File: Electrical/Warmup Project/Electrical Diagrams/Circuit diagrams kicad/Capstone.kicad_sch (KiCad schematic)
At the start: 15 parts, among them M2 Motor_DC, U2 MCP2561-E-MF, U3 OP AMP, U4 INA125P

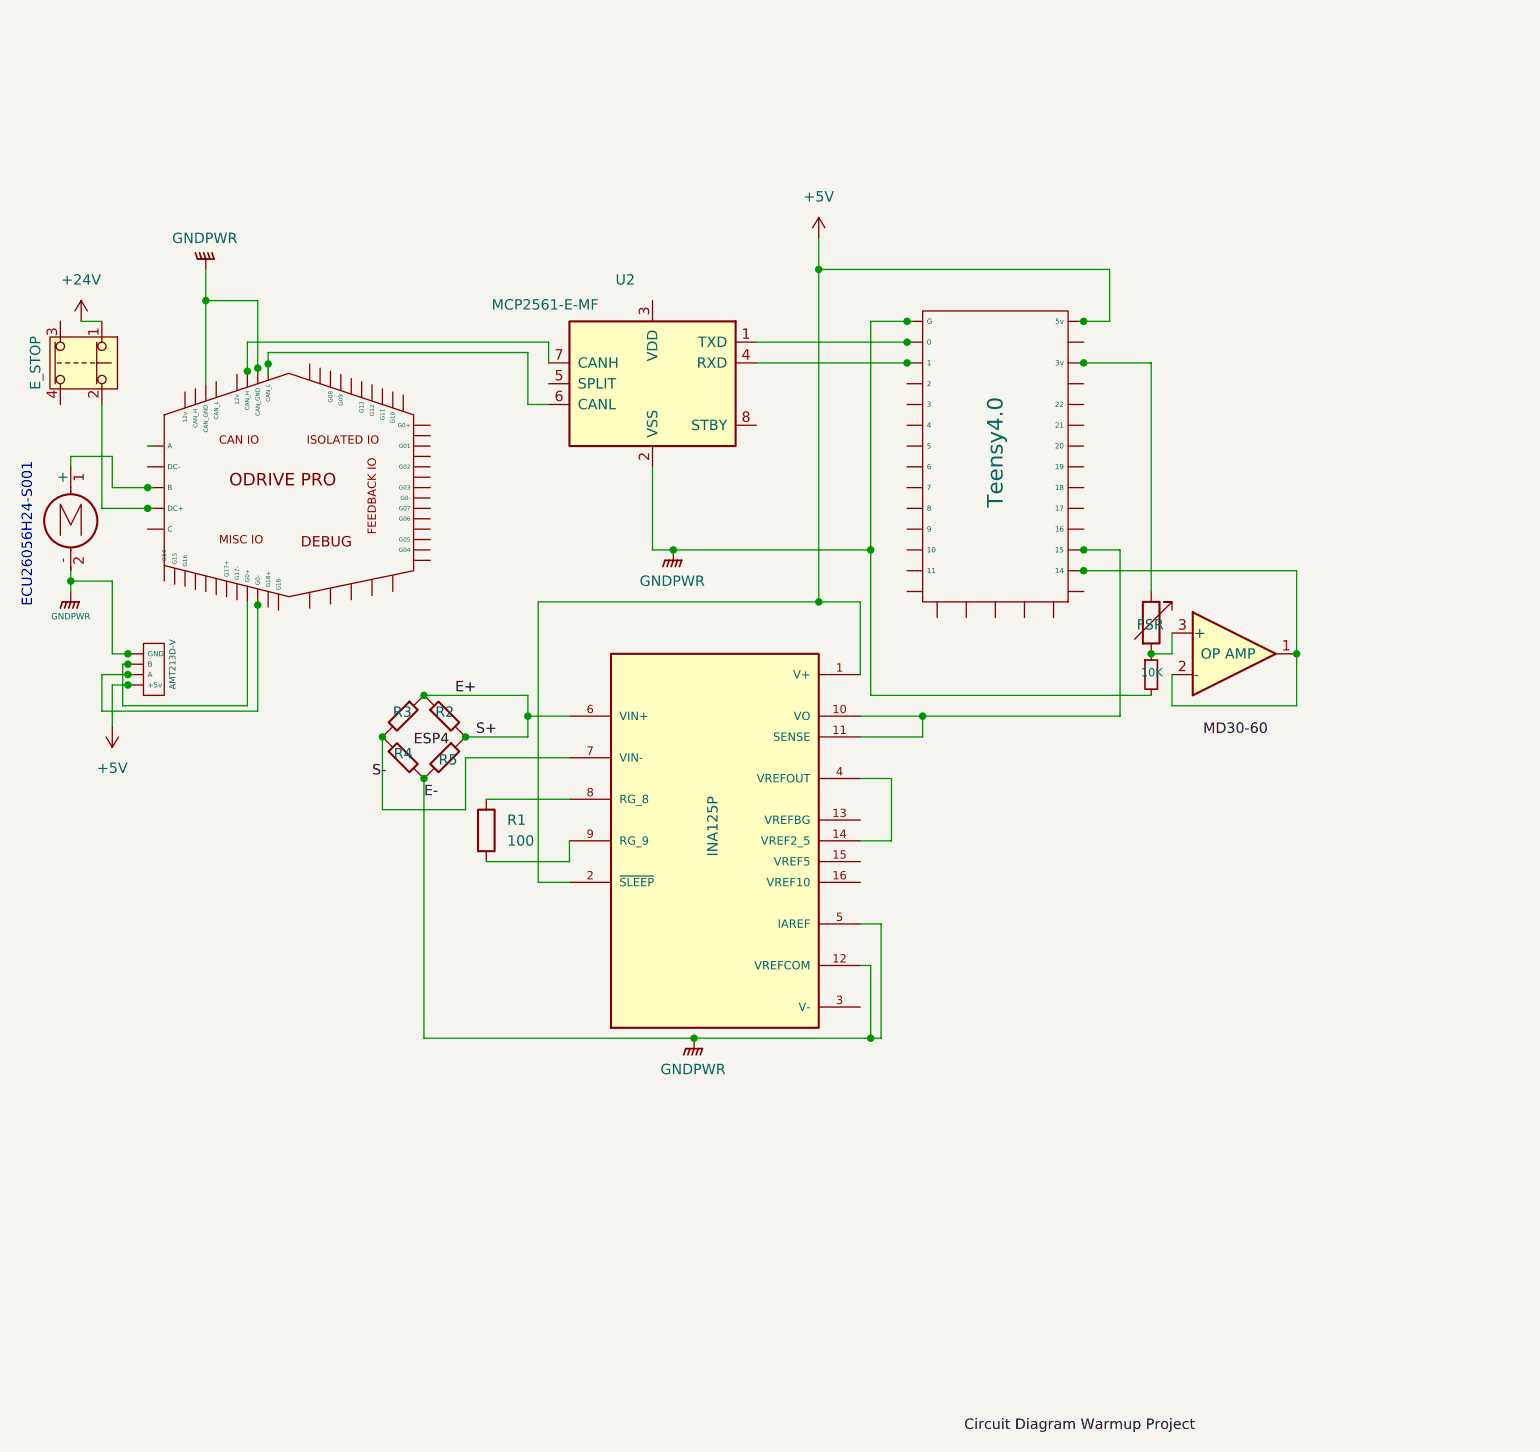
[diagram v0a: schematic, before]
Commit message: Updated code
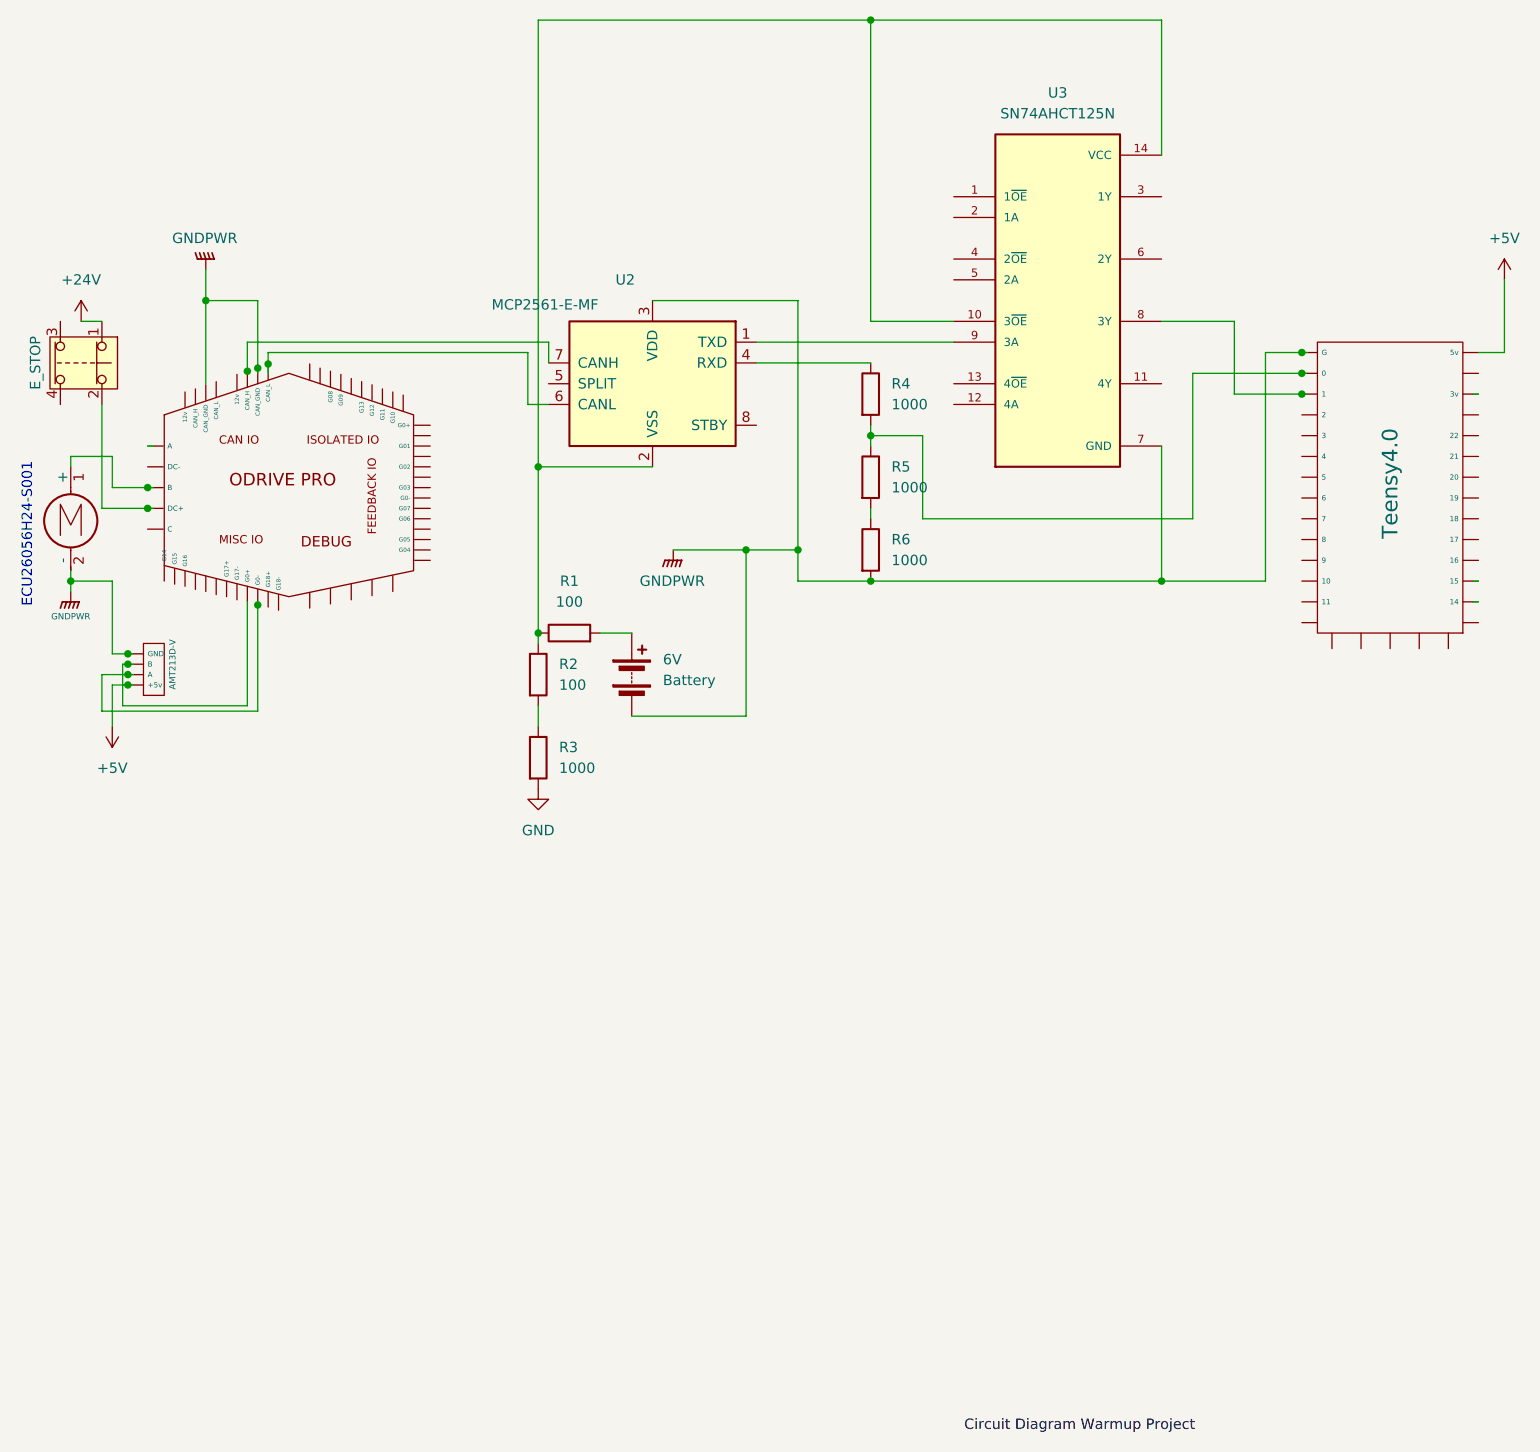
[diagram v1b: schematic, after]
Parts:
- removed 10K: R_Small, symbol Device:R_Small
- removed FSR: R_Variable, symbol Device:R_Variable
- removed R2, R3, R4, R5: R_45deg, symbol Device:R_45deg
- removed U3: OP AMP, Package_SO:VSSOP-8_3x3mm_P0.65mm, symbol Amplifier_Operational:OPA1662DGK
- removed U4: INA125P, DIP794W45P254L1969H508Q16, symbol INA125P:INA125P
- added 6V: Battery, symbol Device:Battery
- added R2: 100, symbol Device:R
- added R3, R4, R5, R6: 1000, symbol Device:R
- added U3: SN74AHCT125N, SN74AHCT125N:DIP794W45P254L1930H508Q14, symbol SN74AHCT125N:SN74AHCT125N
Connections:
- net GNDPWR: now also U2.3 (VDD), 6V.2 (-), R6.2, U3.7 (GND); no longer U2.2 (VSS), U2.9 (VSS)
- net at R1.1: now also U2.2 (VSS), U2.9 (VSS), R2.1, U3.10 (3~{OE}), U3.14 (VCC)
- net at R1.2: now also 6V.1 (+)
- net at U2.1 (TXD): now also U3.9 (3A); no longer Teensy4.0. (G)
- net at U2.4 (RXD): now also R4.1; no longer Teensy4.0. (G)
- new net: R4.2, R5.1, Teensy4.0. (G)
- new net: R2.2, R3.1
- new net: R5.2, R6.1
- new net: Teensy4.0. (G), U3.8 (3Y)
- new net: AMT213D-V. (GND), U1. (x2)
- new net GND: R3.2
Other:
- moved on the sheet: Teensy4.0
